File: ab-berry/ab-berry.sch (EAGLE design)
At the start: 34 parts, among them U1 LM1117MPX-3.3/NOPB or AP2114H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

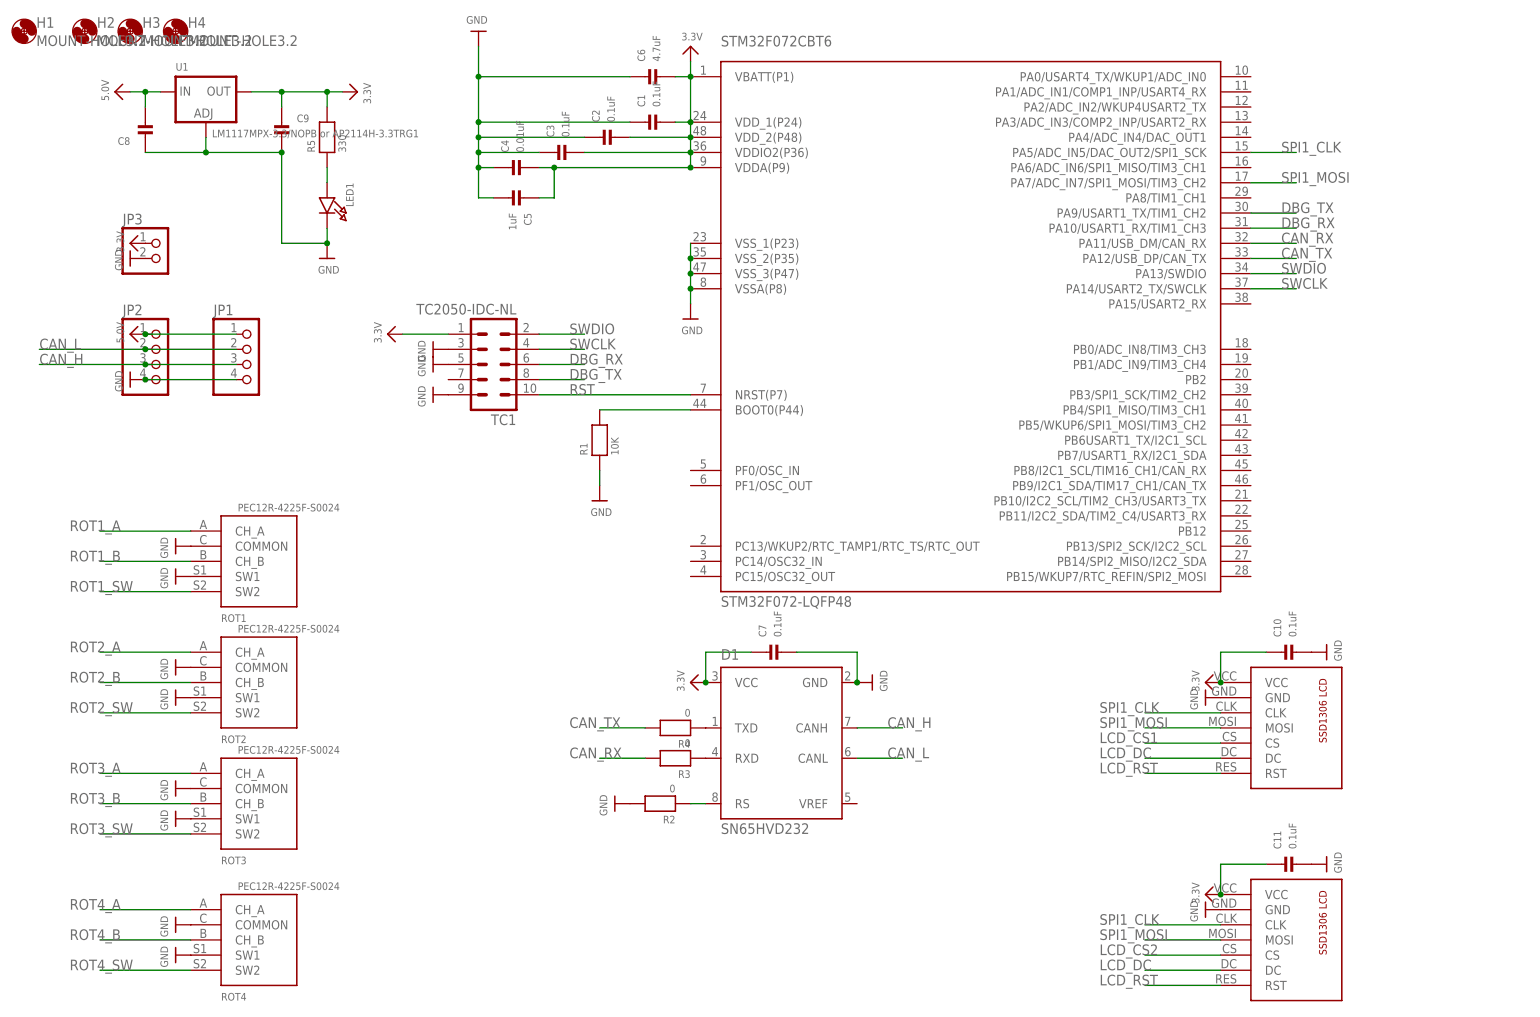
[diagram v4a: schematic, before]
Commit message: ab-berry
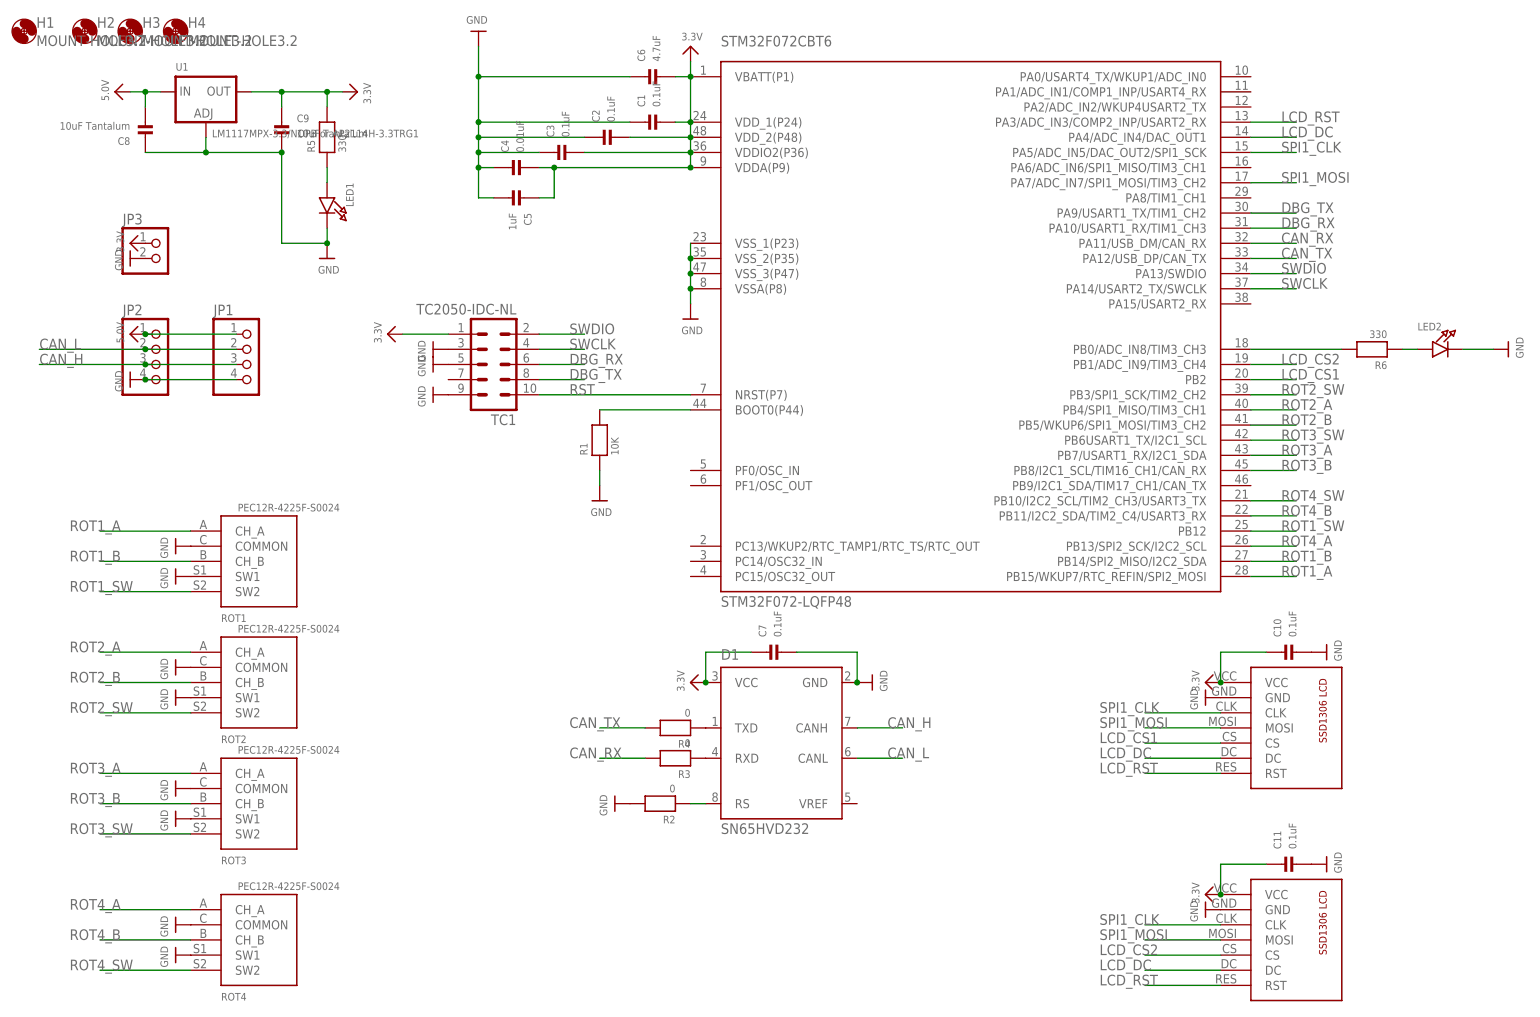
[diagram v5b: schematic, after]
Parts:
- added LED2: (no value), microbuilder:LED0603
- added R6: 330, microbuilder:RESISTOR0603
- C8, C9: value (none) -> 10uF Tantalum
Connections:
- new net N$6: R6.2, STM32F072CBT6.PB0/ADC_IN8/TIM3_CH3
- new net N$7: LED2.A, R6.1
- net GND: now also LED2.C
- net LCD_CS1: now also STM32F072CBT6.PB2
- net LCD_CS2: now also STM32F072CBT6.PB1/ADC_IN9/TIM3_CH4
- net LCD_DC: now also STM32F072CBT6.PA4/ADC_IN4/DAC_OUT1
- net LCD_RST: now also STM32F072CBT6.PA3/ADC_IN3/COMP2_INP/USART2_RX
- net ROT1_A: now also STM32F072CBT6.PB15/WKUP7/RTC_REFIN/SPI2_MOSI
- net ROT1_B: now also STM32F072CBT6.PB14/SPI2_MISO/I2C2_SDA
- net ROT1_SW: now also STM32F072CBT6.PB12
- net ROT2_A: now also STM32F072CBT6.PB4/SPI1_MISO/TIM3_CH1
- net ROT2_B: now also STM32F072CBT6.PB5/WKUP6/SPI1_MOSI/TIM3_CH2
- net ROT2_SW: now also STM32F072CBT6.PB3/SPI1_SCK/TIM2_CH2
- net ROT3_A: now also STM32F072CBT6.PB7/USART1_RX/I2C1_SDA
- net ROT3_B: now also STM32F072CBT6.PB8/I2C1_SCL/TIM16_CH1/CAN_RX
- net ROT3_SW: now also STM32F072CBT6.PB6USART1_TX/I2C1_SCL
- net ROT4_A: now also STM32F072CBT6.PB13/SPI2_SCK/I2C2_SCL
- net ROT4_B: now also STM32F072CBT6.PB11/I2C2_SDA/TIM2_C4/USART3_RX
- net ROT4_SW: now also STM32F072CBT6.PB10/I2C2_SCL/TIM2_CH3/USART3_TX

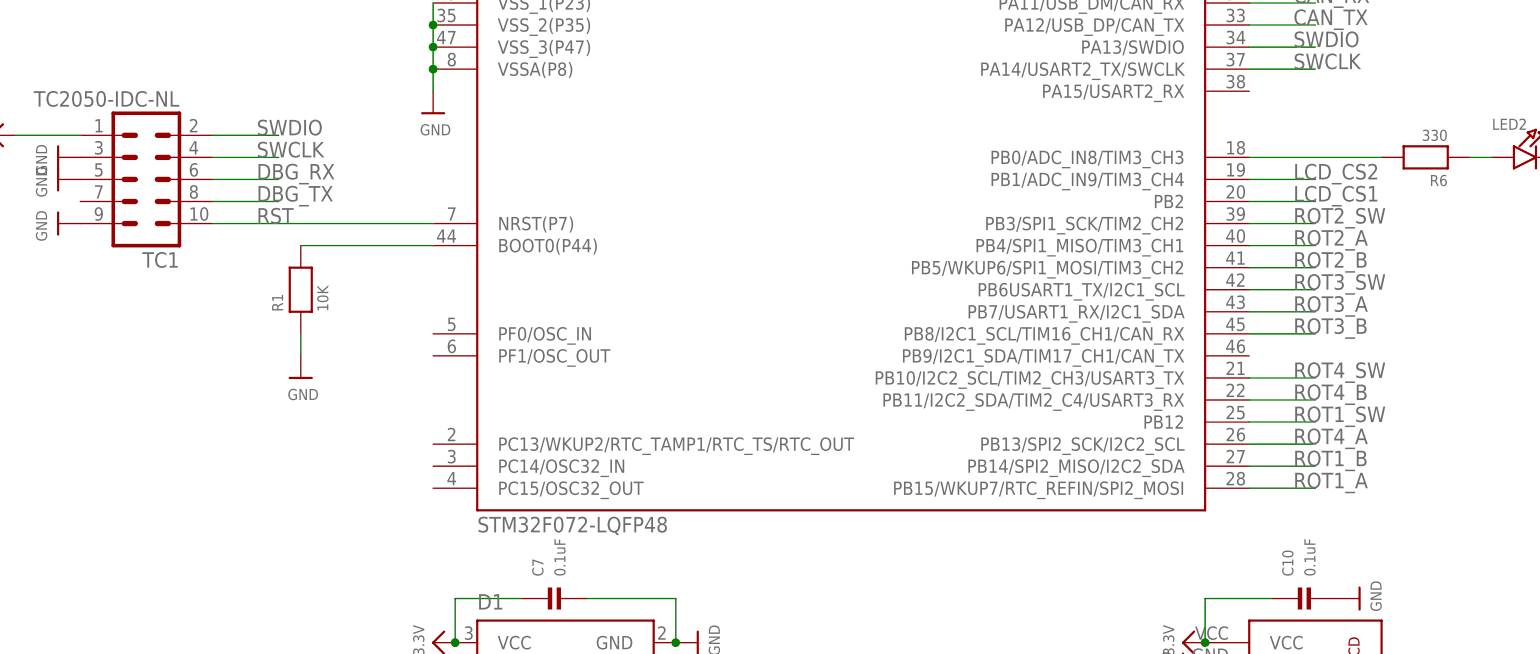
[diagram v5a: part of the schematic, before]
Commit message: ab-berry: added xtal :/
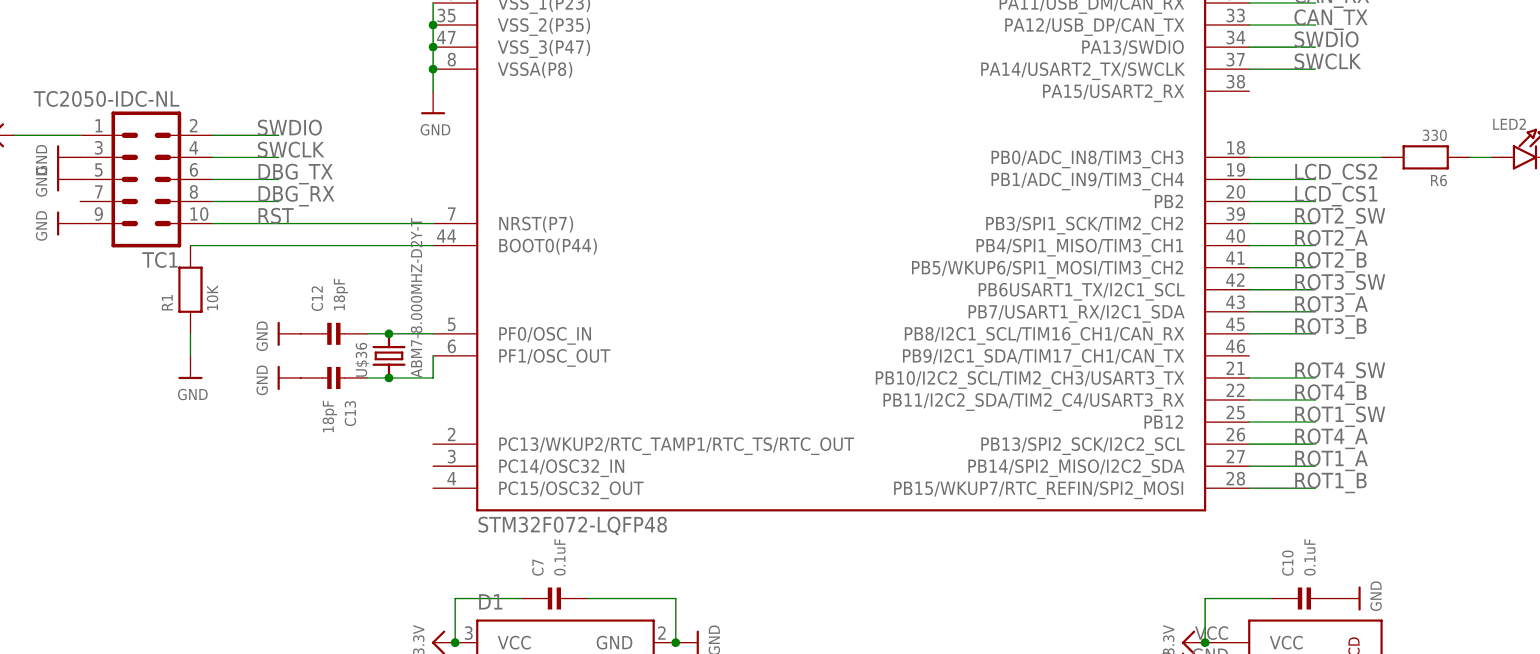
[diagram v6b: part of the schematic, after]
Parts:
- added C12, C13: 18pF, microbuilder:CAP_CERAMIC0603
- added U$36: ABM7-8.000MHZ-D2Y-T, keves:ABM7-8.000MHZ-D2Y-T
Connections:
- new net N$8: C12.P$2, STM32F072CBT6.PF0/OSC_IN, U$36.2
- new net N$9: C13.P$1, STM32F072CBT6.PF1/OSC_OUT, U$36.1
- net DBG_RX: now also TC1.8; no longer TC1.6
- net DBG_TX: now also TC1.6; no longer TC1.8
- net GND: now also C12.P$1, C13.P$2
- net ROT1_A: now also STM32F072CBT6.PB14/SPI2_MISO/I2C2_SDA; no longer STM32F072CBT6.PB15/WKUP7/RTC_REFIN/SPI2_MOSI
- net ROT1_B: now also STM32F072CBT6.PB15/WKUP7/RTC_REFIN/SPI2_MOSI; no longer STM32F072CBT6.PB14/SPI2_MISO/I2C2_SDA
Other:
- moved on the sheet: R1
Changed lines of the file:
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@@
 <?xml version="1.0" encoding="utf-8"?>
 <!DOCTYPE eagle SYSTEM "eagle.dtd">
-<eagle version="7.5.0">
+<eagle version="7.2.0">
 <drawing>
 <settings>
@@
 <part name="LED2" library="microbuilder" deviceset="LED" device="0603"/>
 <part name="U$33" library="microbuilder" deviceset="GND" device=""/>
+<part name="C12" library="microbuilder" deviceset="CAP_CERAMIC" device="0603" value="18pF"/>
+<part name="C13" library="microbuilder" deviceset="CAP_CERAMIC" device="0603" value="18pF"/>
+<part name="U$34" library="microbuilder" deviceset="GND" device=""/>
+<part name="U$35" library="microbuilder" deviceset="GND" device=""/>
+<part name="U$36" library="keves" deviceset="ABM7-8.000MHZ-D2Y-T" device=""/>
 </parts>
 <sheets>
@@
 <instance part="U$7" gate="G$1" x="-20.32" y="38.1" rot="R270"/>
 <instance part="U$8" gate="G$1" x="-20.32" y="33.02" rot="R270"/>
-<instance part="R1" gate="G$1" x="7.62" y="25.4" rot="R90"/>
-<instance part="U$4" gate="G$1" x="7.62" y="15.24"/>
+<instance part="R1" gate="G$1" x="-5.08" y="25.4" rot="R90"/>
+<instance part="U$4" gate="G$1" x="-5.08" y="15.24"/>
 <instance part="D1" gate="G$1" x="38.1" y="-25.4"/>
 <instance part="R2" gate="G$1" x="17.78" y="-35.56" rot="R180"/>
@@
 <instance part="LED2" gate="G$1" x="149.86" y="40.64"/>
 <instance part="U$33" gate="G$1" x="160.02" y="40.64" rot="R90"/>
+<instance part="C12" gate="G$1" x="12.7" y="20.32" rot="R90"/>
+<instance part="C13" gate="G$1" x="10.16" y="15.24" rot="R270"/>
+<instance part="U$34" gate="G$1" x="5.08" y="15.24" rot="R270"/>
+<instance part="U$35" gate="G$1" x="5.08" y="20.32" rot="R270"/>
+<instance part="U$36" gate="G$1" x="17.78" y="17.78" rot="R90"/>
 </instances>
 <busses>
@@
 <pinref part="R1" gate="G$1" pin="1"/>
 <pinref part="U$4" gate="G$1" pin="GND"/>
-<wire x1="7.62" y1="17.78" x2="7.62" y2="20.32" width="0.1524" layer="91"/>
+<wire x1="-5.08" y1="17.78" x2="-5.08" y2="20.32" width="0.1524" layer="91"/>
 </segment>
 <segment>
@@
 <pinref part="U$33" gate="G$1" pin="GND"/>
 <wire x1="157.48" y1="40.64" x2="152.4" y2="40.64" width="0.1524" layer="91"/>
+</segment>
+<segment>
+<pinref part="C13" gate="G$1" pin="P$2"/>
+<pinref part="U$34" gate="G$1" pin="GND"/>
+</segment>
+<segment>
+<pinref part="C12" gate="G$1" pin="P$1"/>
+<pinref part="U$35" gate="G$1" pin="GND"/>
 </segment>
 </net>
@@
 <net name="DBG_TX" class="0">
 <segment>
+<pinref part="STM32F072CBT6" gate="G$1" pin="PA9/USART1_TX/TIM1_CH2"/>
+<wire x1="116.84" y1="63.5" x2="124.46" y2="63.5" width="0.1524" layer="91"/>
+<label x="121.92" y="63.5" size="1.778" layer="95"/>
+</segment>
+<segment>
+<pinref part="TC1" gate="A" pin="6"/>
+<wire x1="-2.54" y1="38.1" x2="5.08" y2="38.1" width="0.1524" layer="91"/>
+<label x="2.54" y="38.1" size="1.778" layer="95"/>
+</segment>
+</net>
+<net name="DBG_RX" class="0">
+<segment>
+<pinref part="STM32F072CBT6" gate="G$1" pin="PA10/USART1_RX/TIM1_CH3"/>
+<wire x1="116.84" y1="60.96" x2="124.46" y2="60.96" width="0.1524" layer="91"/>
+<label x="121.92" y="60.96" size="1.778" layer="95"/>
+</segment>
+<segment>
 <pinref part="TC1" gate="A" pin="8"/>
 <wire x1="-2.54" y1="35.56" x2="5.08" y2="35.56" width="0.1524" layer="91"/>
 <label x="2.54" y="35.56" size="1.778" layer="95"/>
 </segment>
-<segment>
-<pinref part="STM32F072CBT6" gate="G$1" pin="PA9/USART1_TX/TIM1_CH2"/>
-<wire x1="116.84" y1="63.5" x2="124.46" y2="63.5" width="0.1524" layer="91"/>
-<label x="121.92" y="63.5" size="1.778" layer="95"/>
-</segment>
-</net>
-<net name="DBG_RX" class="0">
-<segment>
-<pinref part="STM32F072CBT6" gate="G$1" pin="PA10/USART1_RX/TIM1_CH3"/>
-<wire x1="116.84" y1="60.96" x2="124.46" y2="60.96" width="0.1524" layer="91"/>
-<label x="121.92" y="60.96" size="1.778" layer="95"/>
-</segment>
-<segment>
-<pinref part="TC1" gate="A" pin="6"/>
-<wire x1="-2.54" y1="38.1" x2="5.08" y2="38.1" width="0.1524" layer="91"/>
-<label x="2.54" y="38.1" size="1.778" layer="95"/>
-</segment>
 </net>
 <net name="N$1" class="0">
@@
 <pinref part="STM32F072CBT6" gate="G$1" pin="BOOT0(P44)"/>
 <pinref part="R1" gate="G$1" pin="2"/>
-<wire x1="22.86" y1="30.48" x2="7.62" y2="30.48" width="0.1524" layer="91"/>
+<wire x1="22.86" y1="30.48" x2="-5.08" y2="30.48" width="0.1524" layer="91"/>
 </segment>
 </net>
@@
 </segment>
 <segment>
+<pinref part="STM32F072CBT6" gate="G$1" pin="PB14/SPI2_MISO/I2C2_SDA"/>
+<wire x1="116.84" y1="5.08" x2="124.46" y2="5.08" width="0.1524" layer="91"/>
+<label x="121.92" y="5.08" size="1.778" layer="95"/>
+</segment>
+</net>
+<net name="ROT1_B" class="0">
+<segment>
+<pinref part="ROT1" gate="G$1" pin="CH_B"/>
+<wire x1="-60.96" y1="5.08" x2="-76.2" y2="5.08" width="0.1524" layer="91"/>
+<label x="-81.28" y="5.08" size="1.778" layer="95"/>
+</segment>
+<segment>
 <pinref part="STM32F072CBT6" gate="G$1" pin="PB15/WKUP7/RTC_REFIN/SPI2_MOSI"/>
 <wire x1="116.84" y1="2.54" x2="124.46" y2="2.54" width="0.1524" layer="91"/>
@@
 </segment>
 </net>
-<net name="ROT1_B" class="0">
-<segment>
-<pinref part="ROT1" gate="G$1" pin="CH_B"/>
-<wire x1="-60.96" y1="5.08" x2="-76.2" y2="5.08" width="0.1524" layer="91"/>
-<label x="-81.28" y="5.08" size="1.778" layer="95"/>
-</segment>
-<segment>
-<pinref part="STM32F072CBT6" gate="G$1" pin="PB14/SPI2_MISO/I2C2_SDA"/>
-<wire x1="116.84" y1="5.08" x2="124.46" y2="5.08" width="0.1524" layer="91"/>
-<label x="121.92" y="5.08" size="1.778" layer="95"/>
-</segment>
-</net>
 <net name="ROT1_SW" class="0">
 <segment>
@@
 </segment>
 </net>
+<net name="N$8" class="0">
+<segment>
+<pinref part="C12" gate="G$1" pin="P$2"/>
+<pinref part="STM32F072CBT6" gate="G$1" pin="PF0/OSC_IN"/>
+<wire x1="15.24" y1="20.32" x2="17.78" y2="20.32" width="0.1524" layer="91"/>
+<pinref part="U$36" gate="G$1" pin="2"/>
+<wire x1="17.78" y1="20.32" x2="22.86" y2="20.32" width="0.1524" layer="91"/>
+<junction x="17.78" y="20.32"/>
+</segment>
+</net>
+<net name="N$9" class="0">
+<segment>
+<pinref part="C13" gate="G$1" pin="P$1"/>
+<pinref part="STM32F072CBT6" gate="G$1" pin="PF1/OSC_OUT"/>
+<wire x1="15.24" y1="15.24" x2="17.78" y2="15.24" width="0.1524" layer="91"/>
+<wire x1="17.78" y1="15.24" x2="22.86" y2="15.24" width="0.1524" layer="91"/>
+<wire x1="22.86" y1="15.24" x2="22.86" y2="17.78" width="0.1524" layer="91"/>
+<pinref part="U$36" gate="G$1" pin="1"/>
+<junction x="17.78" y="15.24"/>
+</segment>
+</net>
